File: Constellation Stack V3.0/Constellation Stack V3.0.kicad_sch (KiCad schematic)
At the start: 85 parts, among them J1 PWR, J2 PROG SOCKET, J3 PT_IN, J5 CAN_TERMINAL, J7 RS485 Out, J8 GPIO/ESP_ADC OUT, Q2 DMP3099L, SW1 RESET, SW2 GPIO_0, SW3 SW_SPST, U1 AP62150Z6-7, U10 ADS8688, U2 LDK320AM50R, U3 LDL1117S33R, U4 ESP32-PICO-MINI-02U-N8R2, U5 ESP32-WROOM-32UE, U6 BMI088, U7 W25Q16JVSSIQ, U8 MAX485CSA+T, U9 TJA1050T_CM_118

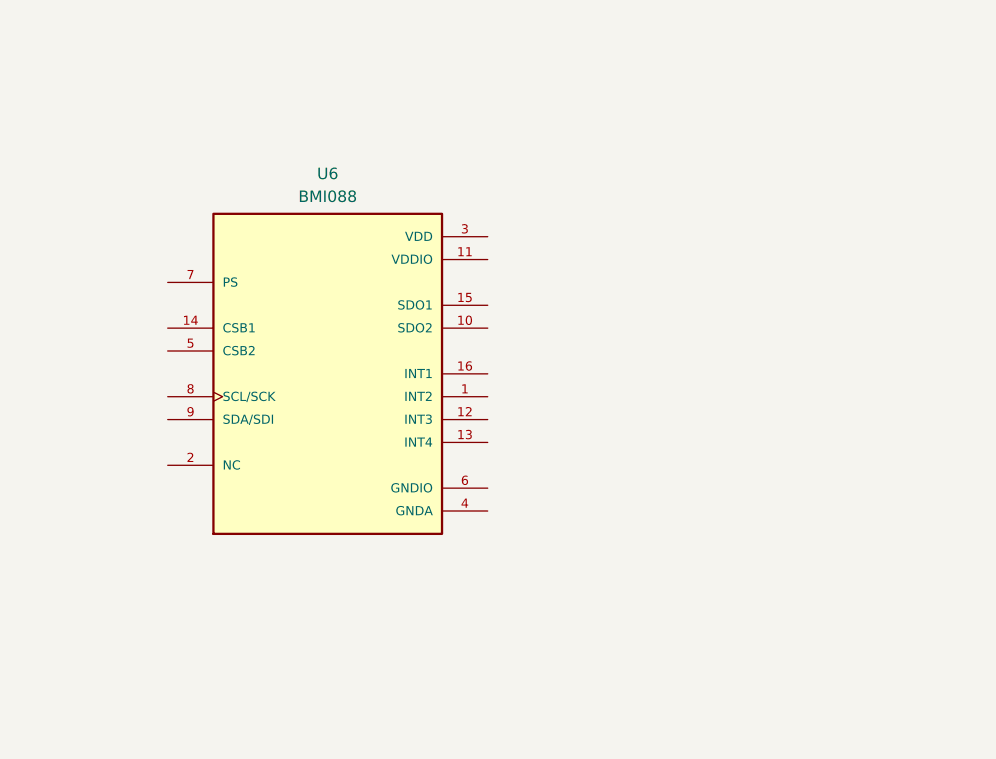
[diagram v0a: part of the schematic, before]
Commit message: 3.0 work
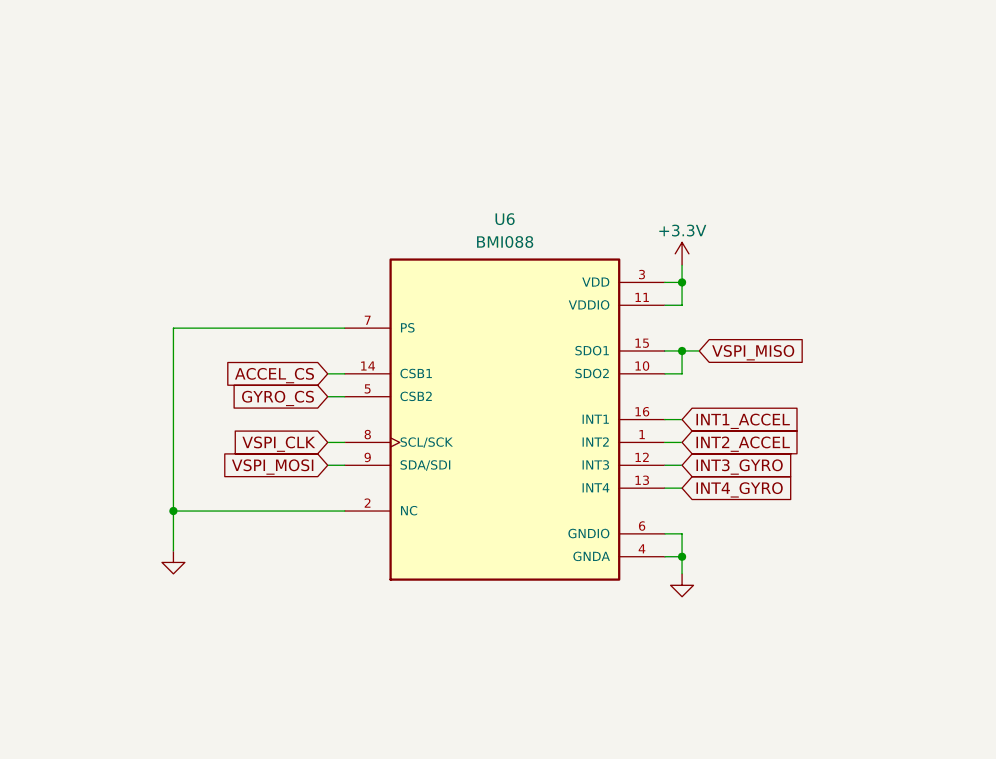
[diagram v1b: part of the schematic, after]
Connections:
- net +3.3V: now also U6.11 (VDDIO), U6.3 (VDD)
- net GND: now also U6.2 (NC), U6.4 (GNDA), U6.6 (GNDIO), U6.7 (PS)
- net VSPI_CLK: now also U6.8 (SCL/SCK)
- net VSPI_MISO: now also U6.10 (SDO2), U6.15 (SDO1)
- net VSPI_MOSI: now also U6.9 (SDA/SDI)
- net INT2_ACCEL: now reaches U6.1 (INT2)
- net INT3_GYRO: now reaches U6.12 (INT3)
- net INT4_GYRO: now reaches U6.13 (INT4)
- net ACCEL_CS: now reaches U6.14 (CSB1)
- net INT1_ACCEL: now reaches U6.16 (INT1)
- net GYRO_CS: now reaches U6.5 (CSB2)
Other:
- moved on the sheet: U6

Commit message: 3.0 stack
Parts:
- removed C22: 1uF, Capacitor_SMD:C_0603_1608Metric, symbol Device:C
- removed C23: 47nf, Capacitor_SMD:C_0603_1608Metric, symbol Device:C_Small
- removed J5: CAN_TERMINAL, Connector_PinSocket_2.54mm:PinSocket_1x02_P2.54mm_Vertical, symbol Connector:Conn_01x02_Socket
- removed R18, R19: 60, Resistor_SMD:R_0805_2012Metric, symbol Device:R_Small
- removed SW3: SW_SPST, Jumper:SolderJumper-2_P1.3mm_Open_RoundedPad1.0x1.5mm, symbol Switch:SW_SPST
- removed TP17, TP18, TP19, TP20: TestPoint, TestPoint:TestPoint_Loop_D2.60mm_Drill1.6mm_Beaded, symbol Connector:TestPoint
- removed U4: ESP32-PICO-MINI-02U-N8R2, ESP32-PICO-MINI-02U:MODULE_ESP32-PICO-MINI-02U-N8R2, symbol ESP32-PICO-MINI-02U:ESP32-PICO-MINI-02U-N8R2
- removed U9: TJA1050T_CM_118, Package_SO:SOIC-8_3.9x4.9mm_P1.27mm, symbol TJA1050T:TJA1050T_CM_118
- added C11, C12, C15, C16: 100nF, Capacitor_SMD:C_0603_1608Metric, symbol Device:C
- added U4: BMP390, BMP390:10LGA_2X2X0p75_BOS, symbol BMP390:BMP390
- SW1, SW2: footprint PTS636SM50JSMTR LFS:SW_PTS636_CNK -> pt36:SW_PTS636_CNK
- U6: footprint BMI088:PQFN50P450X300X100-16N -> bmi088:BMI088
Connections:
- net +3.3V: now also C11.1, C12.1, C15.1, C16.1, U4.1 (VDDIO), U4.10 (VDD)
- net GND: now also C11.2, C12.2, C15.2, C16.2, U4.3 (VSS), U4.8 (VSS), U4.9 (VSS)
- net RXD0: now also J2.2 (Pin_2); no longer J2.3 (Pin_3)
- net TXD0: now also J2.3 (Pin_3); no longer J2.2 (Pin_2)
- net VSPI_CLK: now also U4.2 (SCK)
- net VSPI_MISO: now also U4.5 (SDO)
- net VSPI_MOSI: now also U4.4 (SDI)
- net INT1_ACCEL: no longer names the net of U6.16 (INT1)
- net INT2_ACCEL: no longer names the net of U6.1 (INT2)
- net INT3_GYRO: no longer names the net of U6.12 (INT3)
- net INT4_GYRO: no longer names the net of U6.13 (INT4)
- new net BARO_CS: U4.6 (CSB)
- no-connect marks 6 -> 10
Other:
- note added: "BMI 088 Interial Measurement Unit (IMU)"
- note added: "BMI 390 Barometer"
- note added: "VDD/VDDIO CAPS"
- note removed: "CAN BUS"
- note removed: "TJA1050 CAN Transceiver"
- moved on the sheet: U5, U6

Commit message: 3.0 work
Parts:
- removed J7: RS485 Out, Connector_PinSocket_2.54mm:PinSocket_1x03_P2.54mm_Vertical, symbol Connector:Conn_01x03_Socket
- J1: footprint Connector_PinSocket_2.54mm:PinSocket_1x02_P2.54mm_Vertical -> Connector_PinSocket_2.54mm:PinSocket_1x08_P2.54mm_Vertical; symbol Connector:Conn_01x02_Socket -> Connector:Conn_01x08_Socket
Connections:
- net A: now also J1.6 (Pin_6)
- net B: now also J1.7 (Pin_7)
- net GND: now also J1.8 (Pin_8)
- new net BATT_PWR_SENSE: J1.4 (Pin_4)
- new net EXT_PWR_SENSE: J1.3 (Pin_3)
- no-connect marks 10 -> 11
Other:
- note added: "PIN SOCKET IN/OUT"
- note removed: "PIN SOCKET OUT"
- moved on the sheet: J3
